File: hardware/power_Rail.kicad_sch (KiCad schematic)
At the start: 18 parts

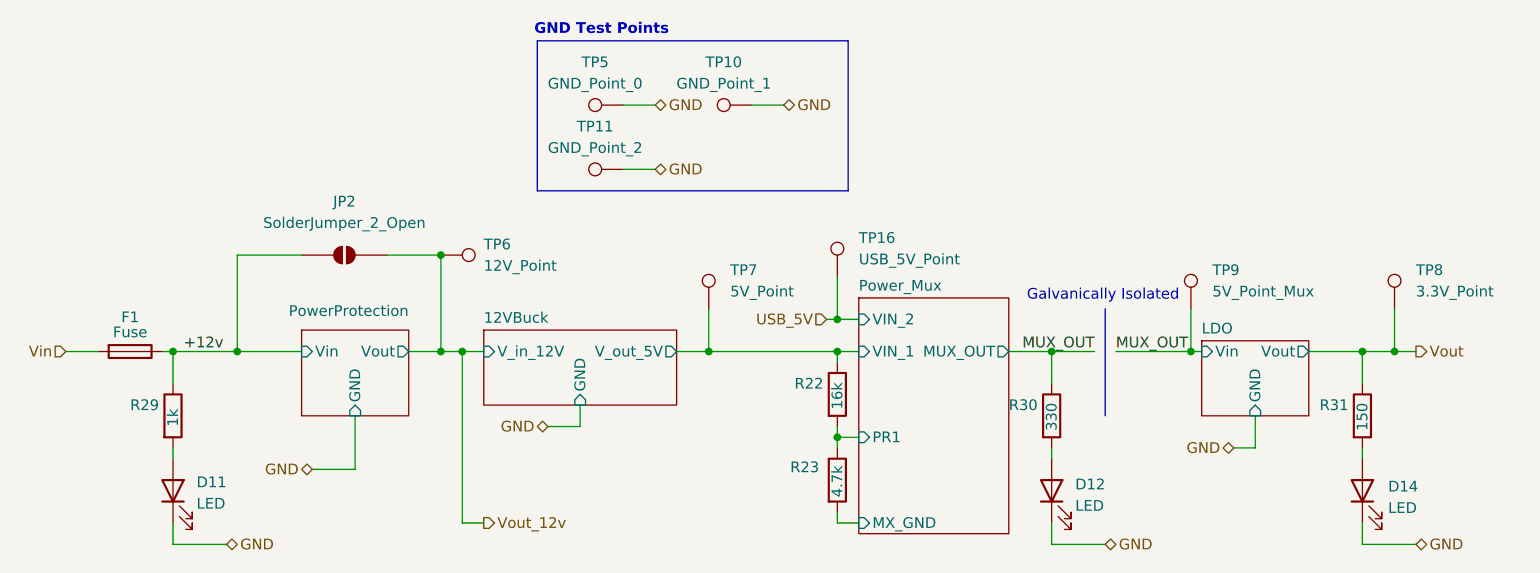
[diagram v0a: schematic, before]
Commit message: Please Final Review
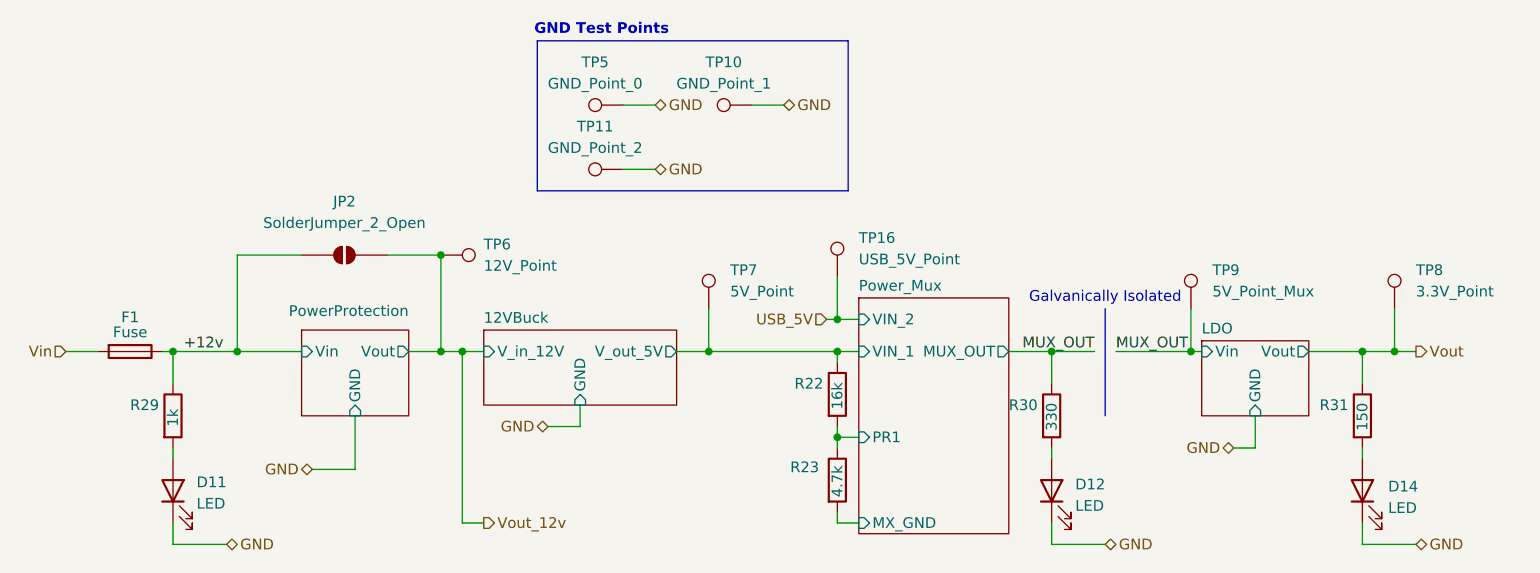
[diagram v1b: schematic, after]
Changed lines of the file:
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@@
 	(text "Galvanically Isolated"
 		(exclude_from_sim no)
-		(at 187.706 74.676 0)
+		(at 187.96 74.93 0)
 		(effects
 			(font
